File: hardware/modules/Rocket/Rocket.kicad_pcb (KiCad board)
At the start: 2 copper layers, 35 x 100 mm, 94 parts, among them J4 Ext Switch, J5 LiPo, J6 Conn_01x02, J8 UFL, SW2 RESET_sw, U10 PCF8563T, U11 SAM-M10Q, U12 E220-900T22S(JP), U14 BMI088, U15 QMC5883L, U2 TPS3820, U4 ESP32-S3-WROOM-1, U5 MCP73871-1CC, U6 INA226, U7 INA226, U8 TPS63070RNMR, U9 INA226, Y2 Crystal

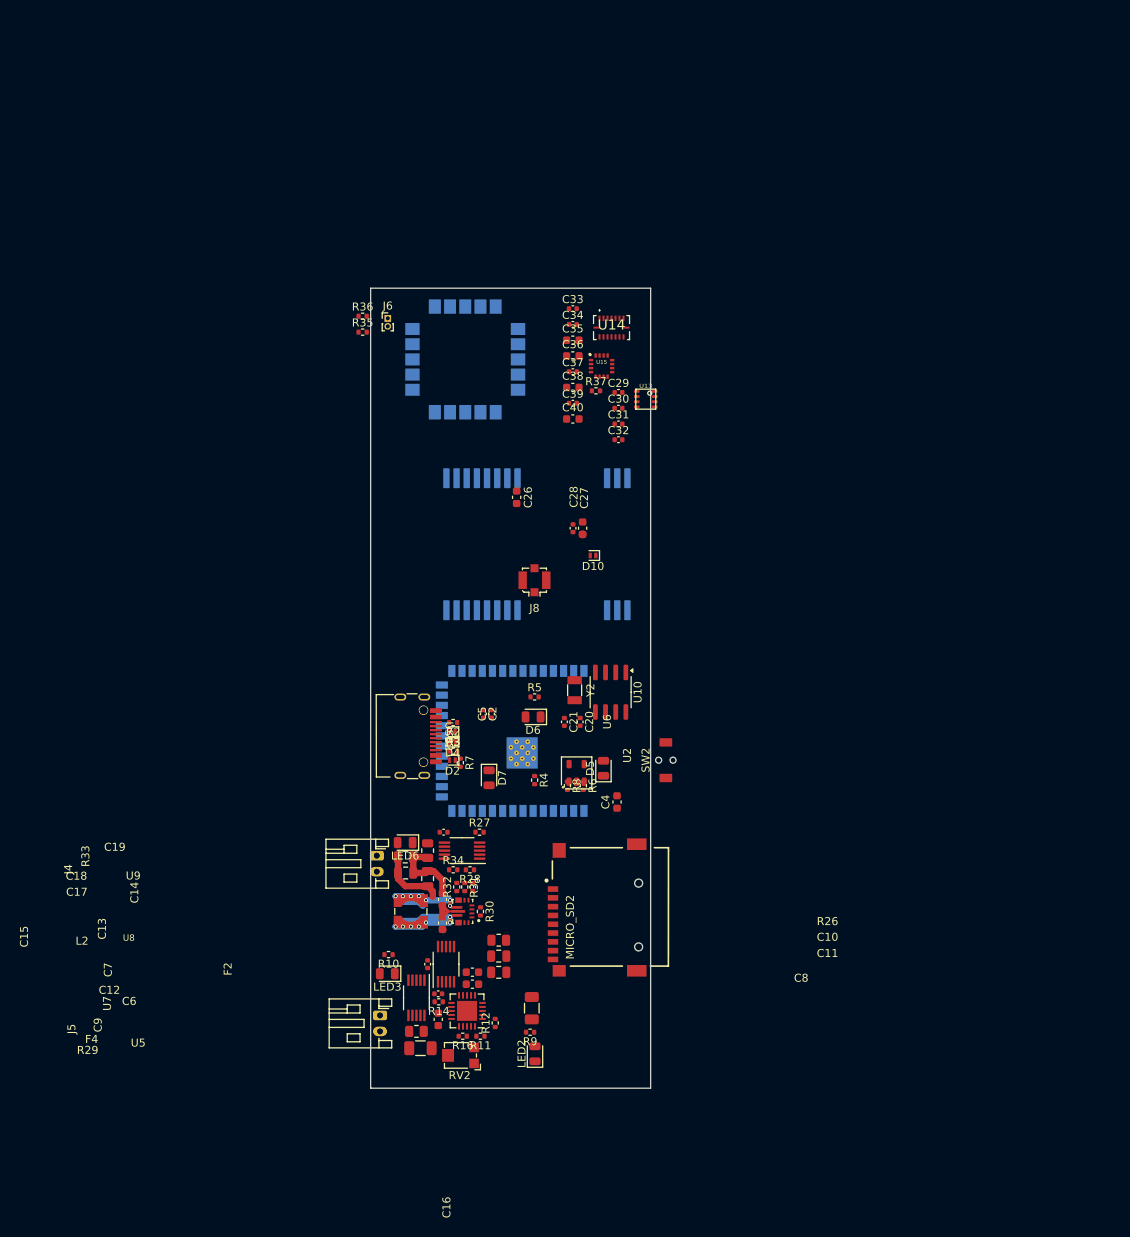
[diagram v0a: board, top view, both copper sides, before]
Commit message: Rocket電装配置
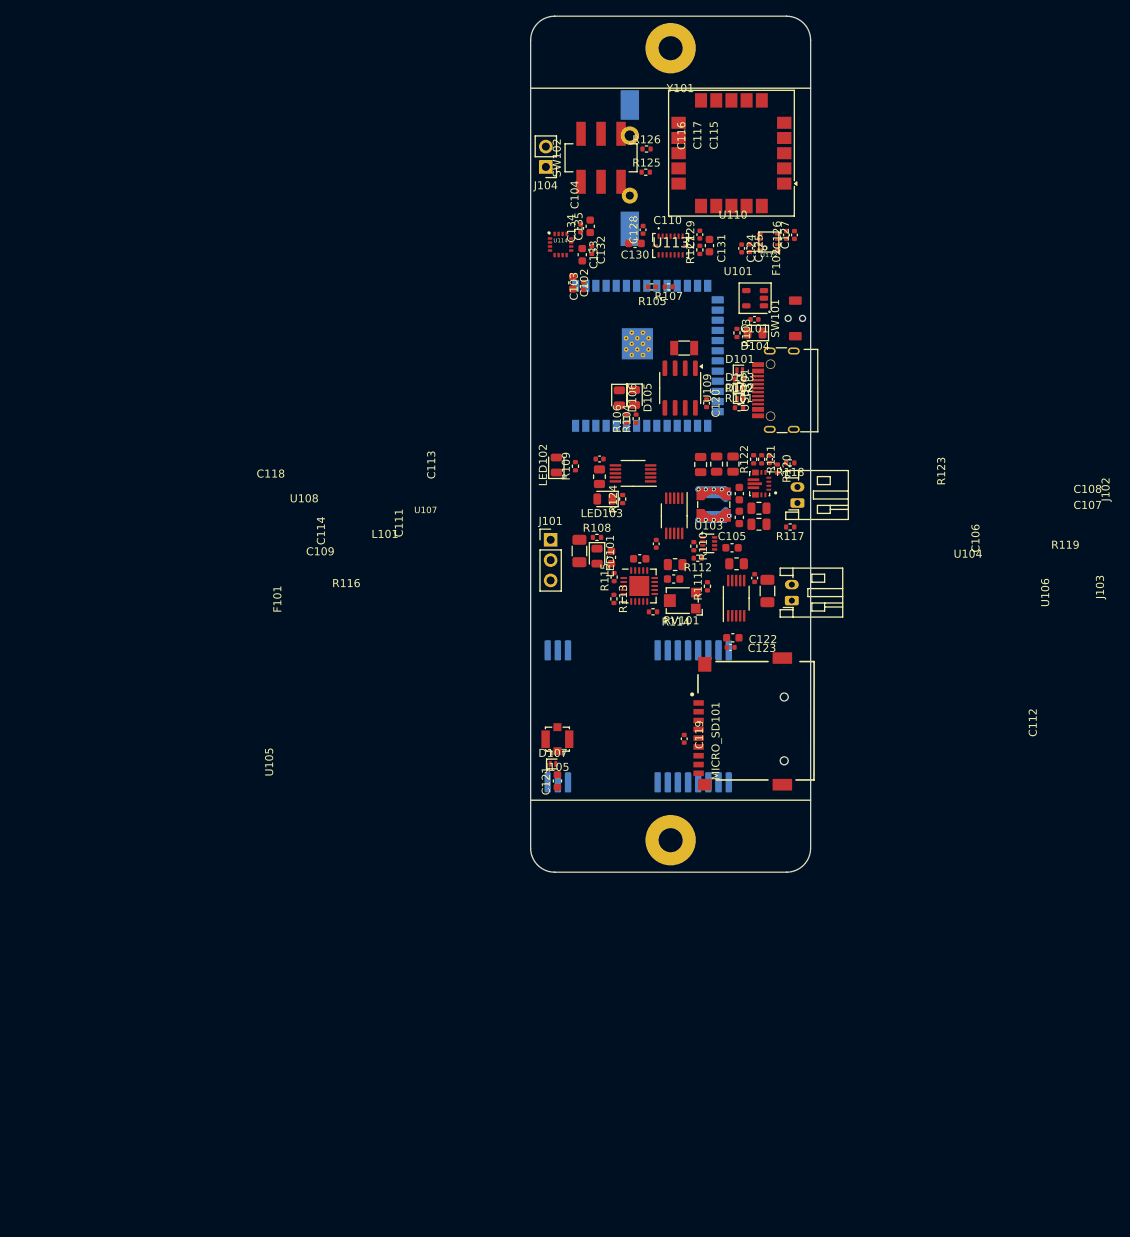
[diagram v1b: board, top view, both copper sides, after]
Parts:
- removed J6: Conn_01x02, Connector_PinHeader_1.00mm:PinHeader_1x02_P1.00mm_Vertical
- added ?: , , F.Cu at (137.5, 47.0)
- added ?: , , F.Cu at (137.5, 146.0)
- added BT101: Battery_Cell, WOBCLibrary:cr1220, B.Cu at (132.4, 61.7)
- added C105: 10uF, Capacitor_SMD:C_0603_1608Metric, F.Cu at (145.2, 109.5)
- added J101: Conn_01x03, Connector_PinHeader_2.54mm:PinHeader_1x03_P2.54mm_Vertical, F.Cu at (122.5, 108.5)
- added J104: Conn_01x02, Connector_PinHeader_2.54mm:PinHeader_1x02_P2.54mm_Vertical, F.Cu at (121.9, 61.8)
- added R110: 4.7k, Resistor_SMD:R_0402_1005Metric, F.Cu at (140.4, 109.2)
- added R112: 10k, Resistor_SMD:R_0402_1005Metric, F.Cu at (140.9, 110.8)
- added SW102: SW_Push_DPDT, WOBCLibrary:IS-2245S-G, F.Cu at (128.8, 60.7)
- added U103: TPS2116DRL, Package_TO_SOT_SMD:SOT-583-8, F.Cu at (142.3, 108.9)
- R101: renamed from R2; value 22k -> 5.1k
- R102: renamed from R3; value 22k -> 5.1k
- U110: renamed from U11; moved to F.Cu
- moved J103 73.1 mm to (152.7, 116.0), turned to 90 degrees
- moved F102 71.7 mm to (149.6, 114.8), turned to -90 degrees
- moved R119 70.8 mm to (145.7, 111.5), turned to 0 degrees
- moved J102 68.6 mm to (153.3, 103.8), turned to 90 degrees
- moved LED102 67.0 mm to (123.2, 99.1), turned to 90 degrees
- moved R120 66.7 mm to (150.8, 99.5)
- moved C108 66.5 mm to (148.5, 104.5)
- moved R109 65.4 mm to (125.6, 99.2), turned to 90 degrees
- moved C112 65.3 mm to (148.0, 113.2), turned to 90 degrees
- moved C102 65.1 mm to (125.3, 76.3), turned to -90 degrees
- moved C113 65.1 mm to (149.9, 98.4)
- moved R121 65.1 mm to (148.9, 98.4)
- moved R122 65.1 mm to (147.9, 98.4)
- moved U107 65.1 mm to (148.6, 101.4)
- moved R118 64.7 mm to (152.4, 98.8)
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- renumbered C2 to C101, C4 to C102, C5 to C103, C6 to C104, C7 to C106, C10 to C107, C11 to C108, C8 to C109, C9 to C110, C13 to C111, C12 to C112, C14 to C113, C15 to C114, C16 to C115, C17 to C116, C18 to C117, C19 to C118, C20 to C119, C21 to C120, C26 to C121, C27 to C122, C28 to C123, C29 to C124, C30 to C125, C31 to C126, C32 to C127, C33 to C128, C34 to C129, C35 to C130, C36 to C131, C37 to C132, C38 to C133, C39 to C134, C40 to C135, D2 to D101, D3 to D102, D4 to D103, D5 to D104, D6 to D105, D7 to D106, D10 to D107, F2 to F101, F4 to F102, J4 to J102, J5 to J103, J8 to J105, L2 to L101, LED2 to LED101, LED3 to LED102, LED6 to LED103, MICRO_SD2 to MICRO_SD101, R4 to R103, R5 to R104, R6 to R105, R7 to R106, R8 to R107, R9 to R108, R10 to R109, R11 to R111, R12 to R113, R14 to R114, R16 to R115, R26 to R116, R27 to R117, R28 to R118, R29 to R119, R30 to R120, R31 to R121, R32 to R122, R33 to R123, R34 to R124, R36 to R125, R35 to R126, R37 to R127, RV2 to RV101, SW2 to SW101, U2 to U101, U4 to U102, U5 to U104, U6 to U105, U7 to U106, U8 to U107, U9 to U108, U10 to U109, U12 to U111, U13 to U112, U14 to U113, U15 to U114, USB2 to USB101, Y2 to Y101
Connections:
- C106 pad 1: Net-(U6-A0) -> VBUS
- C109 pad 1: Net-(U6-Vbus) -> Net-(U103-MODE)
- C112 pad 1: Net-(U6-A0) -> VBUS
- C114 pad 1: /LiPoPower2/VDD_BUS -> VBUS
- C115 pad 1: /LiPoPower2/VDD_BUS -> VBUS
- C116 pad 1: /LiPoPower2/VDD_BUS -> VBUS
- C117 pad 1: /LiPoPower2/VDD_BUS -> VBUS
- C118 pad 1: Net-(U9-VS) -> VBUS
- D101 pad 2: /ESP32Core2/VUSB -> VBUS
- MICRO_SD101 pad 2: /Logger2/SD_SS -> /SS
- MICRO_SD101 pad 3: /Logger2/SD_MOSI -> /MOSI
- MICRO_SD101 pad 5: /Logger2/SD_CLK -> /CLK
- MICRO_SD101 pad 7: /Logger2/SD_MISO -> /MISO
- MICRO_SD101 pad CD1: /Logger2/SD_DET -> /SD_DET
- R105 pad 2: /ESP32Core2/I2C_SCL -> /I2C_SCL
- R107 pad 2: /ESP32Core2/I2C_SDA -> /I2C_SDA
- R109 pad 2: /LiPoPower2/CHARGE_IND -> /CHARGE
- R116 pad 1: Net-(U6-Vbus) -> Net-(U105-Vbus)
- R120 pad 1: /LiPoPower2/VDD_BUS -> VBUS
- R122 pad 2: /LiPoPower2/VDD_BUS -> VBUS
- R123 pad 1: /LiPoPower2/VDD_BUS -> VBUS
- R125 pad 2: /GPS SAM-M10Q2/RX -> Net-(R125-Pad2)
- R126 pad 2: /GPS SAM-M10Q2/TX -> Net-(R126-Pad2)
- U102 pad 10: /ESP32Core2/I2C_SDA -> /I2C_SDA
- U102 pad 11: /ESP32Core2/GPIO18 -> /TimePulse
- U102 pad 12: /ESP32Core2/GPIO8/ADC1_CH7 -> /GPS_RESET
- U102 pad 15: /ESP32Core2/GPIO3/ADC1_CH2 -> /MISO
- U102 pad 20: /ESP32Core2/GPIO12 -> /DetL
- U102 pad 21: /ESP32Core2/GPIO13 -> /ST
- U102 pad 22: /ESP32Core2/GPIO14 -> /CHARGE
- U102 pad 23: /ESP32Core2/GPIO21 -> /PG
- U102 pad 24: /ESP32Core2/GPIO47 -> /STAT1
- U102 pad 25: /ESP32Core2/GPIO48 -> /STAT2
- U102 pad 31: /ESP32Core2/GPIO38 -> /AUX
- U102 pad 32: /ESP32Core2/GPIO39 -> /M0
- U102 pad 33: /ESP32Core2/GPIO40 -> /M1
- U102 pad 36: /ESP32Core2/CAN_RX -> /RTX0
- U102 pad 37: /ESP32Core2/CAN_TX -> /TRX0
- U102 pad 38: /ESP32Core2/GPIO2/ADC1_CH1 -> /SS
- U102 pad 39: /ESP32Core2/GPIO1/ADC1_CH0 -> /CLK
- U102 pad 4: /ESP32Core2/GPIO4/ADC1_CH3 -> /MOSI
- U102 pad 5: /ESP32Core2/GPIO5/ADC1_CH4 -> /SD_DET
- U102 pad 6: /ESP32Core2/GPIO6/ADC1_CH5 -> /TRX1
- U102 pad 7: /ESP32Core2/GPIO7/ADC1_CH6 -> /RTX1
- U102 pad 9: /ESP32Core2/I2C_SCL -> /I2C_SCL
- U104 pad 1: Net-(U6-Vbus) -> Net-(U103-MODE)
- U104 pad 20: Net-(U6-Vbus) -> Net-(U103-MODE)
- U104 pad 6: /LiPoPower2/PG -> /PG
- U104 pad 7: /LiPoPower2/STAT2 -> /STAT2
- U104 pad 8: /LiPoPower2/STAT1 -> /STAT1
- U105 pad 1: /LiPoPower2/I2C_SCL -> /I2C_SCL
- U105 pad 10: Net-(U6-Vbus) -> Net-(U105-Vbus)
- U105 pad 2: Net-(U6-A0) -> VBUS
- U105 pad 4: /LiPoPower2/I2C_SDA -> /I2C_SDA
- U105 pad 5: /LiPoPower2/I2C_SCL -> /I2C_SCL
- U105 pad 6: Net-(U6-A0) -> VBUS
- U105 pad 8: Net-(U6-Vbus) -> Net-(U105-Vbus)
- U106 pad 1: /LiPoPower2/I2C_SCL -> /I2C_SCL
- U106 pad 2: /LiPoPower2/I2C_SCL -> /I2C_SCL
- U106 pad 4: /LiPoPower2/I2C_SDA -> /I2C_SDA
- U106 pad 5: /LiPoPower2/I2C_SCL -> /I2C_SCL
- U106 pad 6: Net-(U6-A0) -> VBUS
- U107 pad 7_8: /LiPoPower2/VDD_BUS -> VBUS
- U108 pad 1: /LiPoPower2/I2C_SCL -> /I2C_SCL
- U108 pad 10: /LiPoPower2/VDD_BUS -> VBUS
- U108 pad 2: /LiPoPower2/I2C_SDA -> /I2C_SDA
- U108 pad 4: /LiPoPower2/I2C_SDA -> /I2C_SDA
- U108 pad 5: /LiPoPower2/I2C_SCL -> /I2C_SCL
- U108 pad 6: Net-(U9-VS) -> VBUS
- U108 pad 8: /LiPoPower2/VDD_BUS -> VBUS
- U109 pad 5: /Logger2/I2C_SDA -> /I2C_SDA
- U109 pad 6: /Logger2/I2C_SCL -> /I2C_SCL
- U110 pad 18: /GPS SAM-M10Q2/RESET -> /GPS_RESET
- U110 pad 7: /GPS SAM-M10Q2/TIME PULSE -> /TimePulse
- U111 pad 5: /LoRa2/LoRa_M0 -> /M0
- U111 pad 6: /LoRa2/LoRa_M1 -> /M1
- U111 pad 7: /LoRa2/LoRa_TRX -> /TRX0
- U111 pad 8: /LoRa2/LoRa_RTX -> /RTX0
- U111 pad 9: /LoRa2/LoRa_AUX -> /AUX
- U112 pad 3: /Pressure2/I2C_SDA -> /I2C_SDA
- U112 pad 4: /Pressure2/I2C_SCL -> /I2C_SCL
- U113 pad 8: /9DoF2/I2C_SCL -> /I2C_SCL
- U113 pad 9: /9DoF2/I2C_SDA -> /I2C_SDA
- U114 pad 1: /9DoF2/I2C_SCL -> /I2C_SCL
- U114 pad 16: /9DoF2/I2C_SDA -> /I2C_SDA
- USB101 pad A4: /ESP32Core2/VUSB -> VBUS
- USB101 pad A9: /ESP32Core2/VUSB -> VBUS
- USB101 pad B4: /ESP32Core2/VUSB -> VBUS
- USB101 pad B9: /ESP32Core2/VUSB -> VBUS
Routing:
- net GND: track 13.3 -> 0.07 mm
- net /LiPoPower2/VDD_BUS: track 9.88 -> 0.00 mm
- net Net-(U107-L1): track 15.9 -> 7.90 mm, vias 7 -> 5
- net Net-(U107-L2): track 12.5 -> 7.90 mm, vias 7 -> 5
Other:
- board size 35 x 100 mm -> 35 x 107 mm
